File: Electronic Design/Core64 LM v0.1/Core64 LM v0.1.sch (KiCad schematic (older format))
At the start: 75 parts, among them J1 PASS THROUGH BOARD, J2 PASS THROUGH BOARD

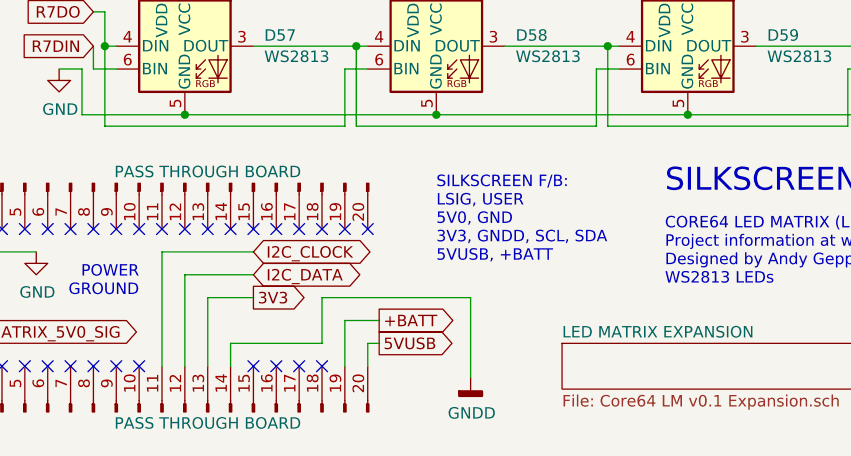
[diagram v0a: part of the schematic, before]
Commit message: Finish layout, revise notes
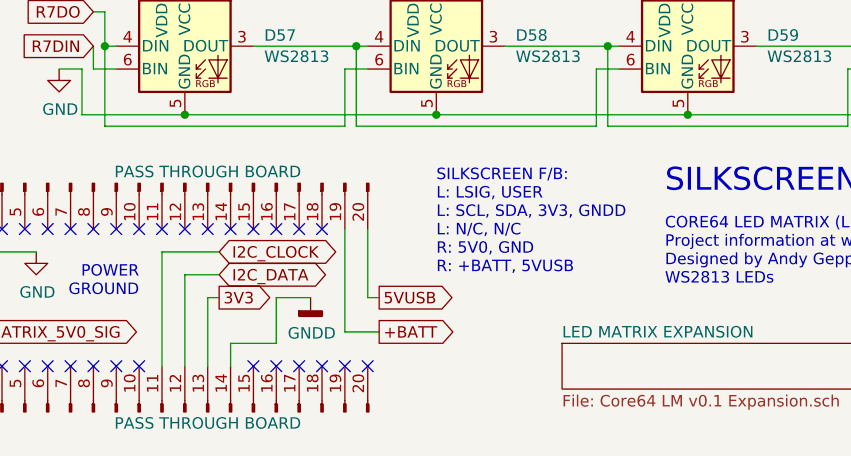
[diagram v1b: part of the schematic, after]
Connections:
- net +BATT: now also J2.19 (Pin_19); no longer J1.19 (Pin_19)
- net 5VUSB: now also J2.20 (Pin_20); no longer J1.20 (Pin_20)
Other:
- note added: "SILKSCREEN F/B:\nL: LSIG, USER\nL: SCL, SDA, 3V3, GNDD\nL: N/C, N/C \nR: 5V0, GND\nR: +BATT, 5VUSB"
- note removed: "SILKSCREEN F/B:\nLSIG, USER\n5V0, GND\n3V3, GNDD, SCL, SDA\n5VUSB, +BATT"
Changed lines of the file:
@@
 Text GLabel 600  7550 2    50   Output ~ 0
 LED_MATRIX_5V0_SIG
-Text Notes 2750 7250 0    50   ~ 0
-SILKSCREEN F/B:\nLSIG, USER\n5V0, GND\n3V3, GNDD, SCL, SDA\n5VUSB, +BATT
+Text Notes 2750 7300 0    50   ~ 0
+SILKSCREEN F/B:\nL: LSIG, USER\nL: SCL, SDA, 3V3, GNDD\nL: N/C, N/C \nR: 5V0, GND\nR: +BATT, 5VUSB
 $Comp
 L Connector:Conn_01x20_Male J2
@@
 Wire Wire Line
 	6000 4450 7100 4450
-Text GLabel 2500 7600 2    50   Output ~ 0
+Text GLabel 2500 7400 2    50   Output ~ 0
 5VUSB
-Text GLabel 2500 7500 2    50   Output ~ 0
+Text GLabel 2500 7550 2    50   Output ~ 0
 +BATT
-NoConn ~ 2350 7100
-NoConn ~ 2450 7100
-Text GLabel 1950 7400 2    50   Output ~ 0
+NoConn ~ 2350 7700
+NoConn ~ 2450 7700
+Text GLabel 1800 7400 2    50   Output ~ 0
 3V3
 Wire Wire Line
@@
 	1750 7700 1750 7400
 Wire Wire Line
-	1750 7400 1950 7400
+	1750 7400 1800 7400
 Wire Wire Line
 	1650 7700 1650 7300
 Wire Wire Line
-	1650 7300 1950 7300
+	1650 7300 1800 7300
 Wire Wire Line
 	1550 7700 1550 7200
 Wire Wire Line
-	1550 7200 1950 7200
-Wire Wire Line
-	2450 7700 2450 7600
-Wire Wire Line
-	2450 7600 2500 7600
-Wire Wire Line
-	2350 7700 2350 7500
-Wire Wire Line
-	2350 7500 2500 7500
+	1550 7200 1800 7200
+Wire Wire Line
+	2450 7100 2450 7400
+Wire Wire Line
+	2450 7400 2500 7400
+Wire Wire Line
+	2350 7100 2350 7550
+Wire Wire Line
+	2350 7550 2500 7550
 $Sheet
 S 3300 7600 1350 200
@@
 F1 "Core64 LM v0.1 Expansion.sch" 50
 $EndSheet
-Text GLabel 1950 7200 2    50   BiDi ~ 0
+Text GLabel 1800 7200 2    50   BiDi ~ 0
 I2C_CLOCK
-Text GLabel 1950 7300 2    50   BiDi ~ 0
+Text GLabel 1800 7300 2    50   BiDi ~ 0
 I2C_DATA
 $Comp
 L power:GNDD #PWR01
 U 1 1 607AD129
-P 2900 7750
-F 0 "#PWR01" H 2900 7500 50  0001 C CNN
-F 1 "GNDD" H 2905 7594 50  0000 C CNN
-F 2 "" H 2900 7750 50  0001 C CNN
-F 3 "" H 2900 7750 50  0001 C CNN
-	1    2900 7750
-	1    0    0    -1
-$EndComp
-Wire Wire Line
-	2900 7750 2900 7400
-Wire Wire Line
-	2900 7400 2250 7400
-Wire Wire Line
-	2250 7400 2250 7600
-Wire Wire Line
-	1850 7600 2250 7600
+P 2200 7400
+F 0 "#PWR01" H 2200 7150 50  0001 C CNN
+F 1 "GNDD" H 2205 7244 50  0000 C CNN
+F 2 "" H 2200 7400 50  0001 C CNN
+F 3 "" H 2200 7400 50  0001 C CNN
+	1    2200 7400
+	1    0    0    -1
+$EndComp
+Wire Wire Line
+	2200 7400 2050 7400
+Wire Wire Line
+	2050 7400 2050 7600
+Wire Wire Line
+	1850 7600 2050 7600
 $EndSCHEMATC
